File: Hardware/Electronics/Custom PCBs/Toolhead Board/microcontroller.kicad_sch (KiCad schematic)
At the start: 34 parts, among them J1 USB C Receptacle, J2 Conn_02x16_Odd_Even, J3 Conn_02x16_Odd_Even, J4 Conn_02x16_Odd_Even, J5 Conn_02x16_Odd_Even, SW1 BOOT, SW2 RESET, U3 RP2040, U4 W25Q128JVS, Y1 12MHz/12pF/50Ω/20ppm

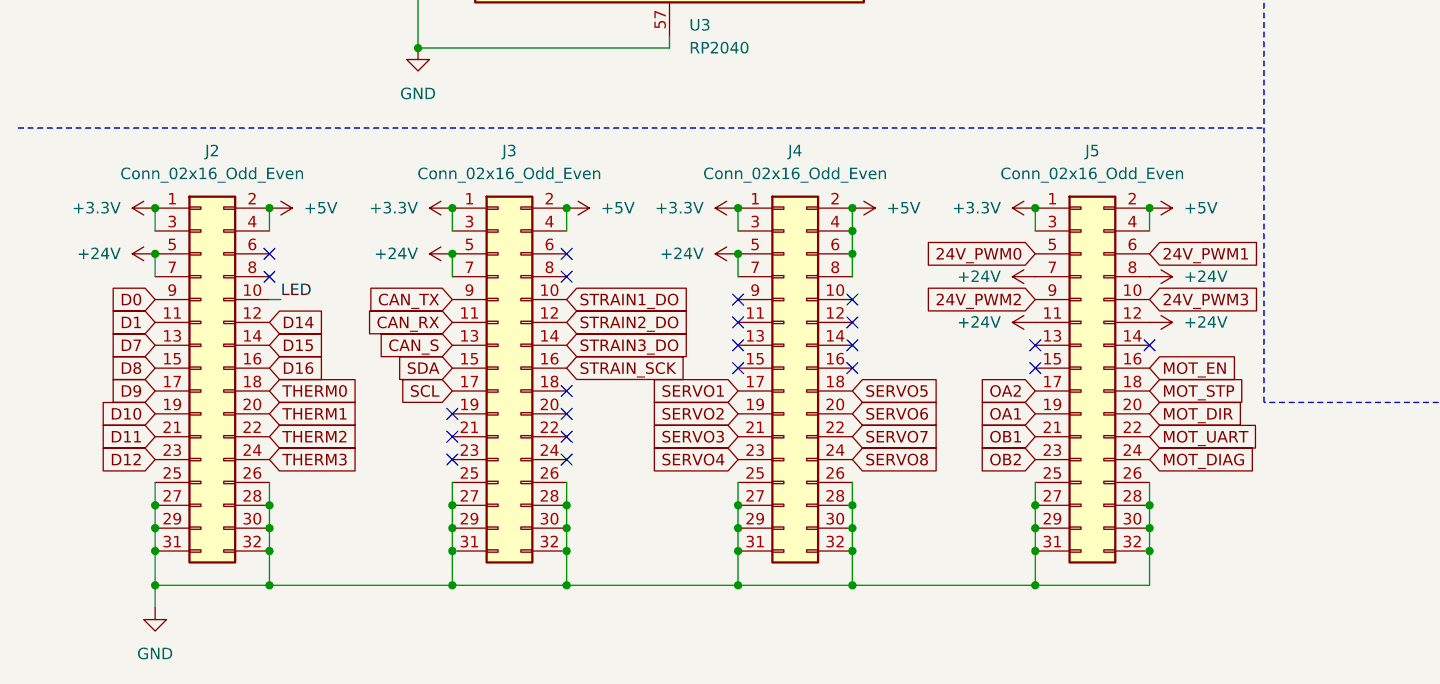
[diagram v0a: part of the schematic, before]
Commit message: Get basic Toolhead Board outline
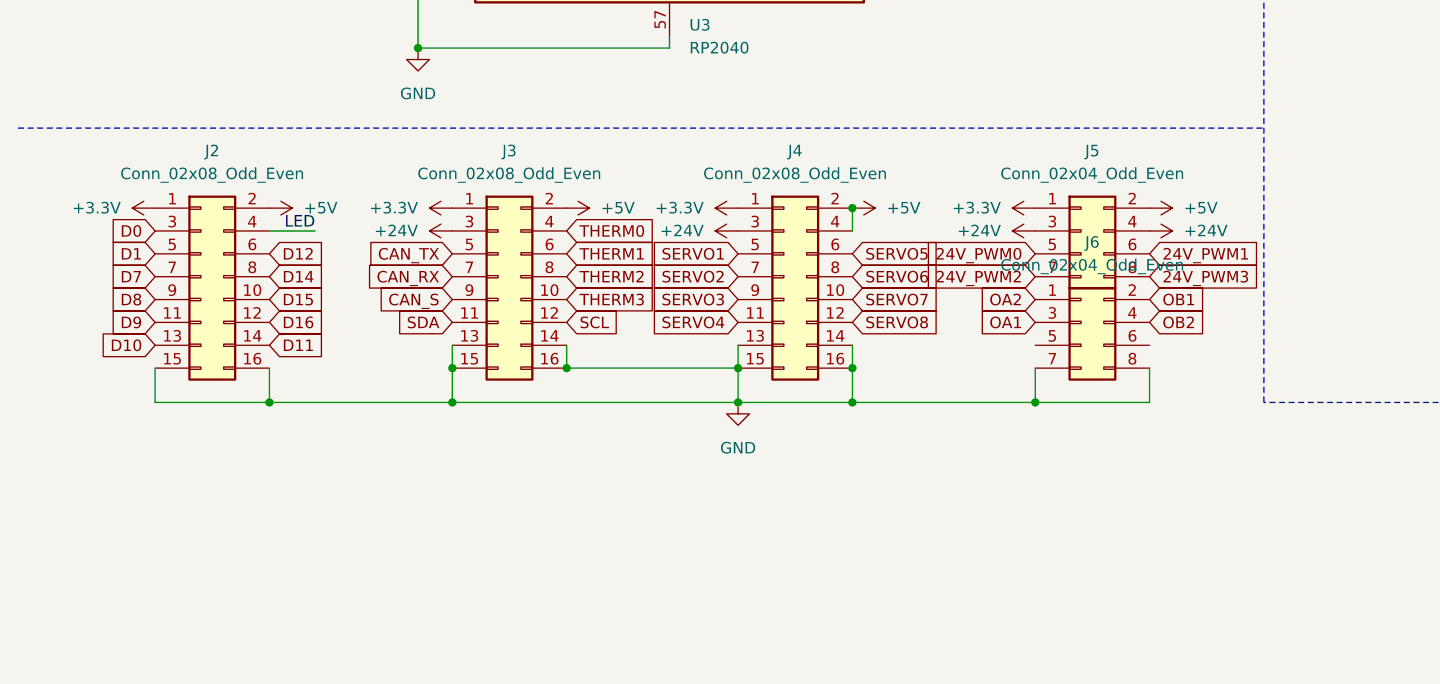
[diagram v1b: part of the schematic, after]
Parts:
- removed J2, J3, J4, J5: Conn_02x16_Odd_Even, Connector_PinHeader_2.54mm:PinHeader_2x16_P2.54mm_Vertical, symbol Connector_Generic:Conn_02x16_Odd_Even
- added J2, J3, J4: Conn_02x08_Odd_Even, Connector_PinSocket_2.54mm:PinSocket_2x08_P2.54mm_Vertical, symbol Connector_Generic:Conn_02x08_Odd_Even
- added J5, J6: Conn_02x04_Odd_Even, Connector_PinSocket_2.54mm:PinSocket_2x04_P2.54mm_Vertical, symbol Connector_Generic:Conn_02x04_Odd_Even
- J1: footprint usb_port:12402012E212A_AMP -> Connector_USB:USB_C_Receptacle_GCT_USB4105-xx-A_16P_TopMnt_Horizontal
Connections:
- net +24V: now also J3.3 (Pin_3), J4.3 (Pin_3), J5.3 (Pin_3), J5.4 (Pin_4)
- net +3.3V: now also J2.1 (Pin_1), J3.1 (Pin_1), J4.1 (Pin_1), J5.1 (Pin_1)
- net +5V: now also J2.2 (Pin_2), J3.2 (Pin_2), J4.2 (Pin_2), J4.4 (Pin_4), J5.2 (Pin_2)
- net 24V_PWM0: now also J5.5 (Pin_5)
- net 24V_PWM1: now also J5.6 (Pin_6)
- net 24V_PWM2: now also J5.7 (Pin_7)
- net 24V_PWM3: now also J5.8 (Pin_8)
- net CAN_RX: now also J3.7 (Pin_7)
- net CAN_S: now also J3.9 (Pin_9)
- net CAN_TX: now also J3.5 (Pin_5)
- net D0: now also J2.3 (Pin_3)
- net D1: now also J2.5 (Pin_5)
- net D10: now also J2.13 (Pin_13)
- net D11: now also J2.14 (Pin_14)
- net D12: now also J2.6 (Pin_6)
- net D14: now also J2.8 (Pin_8)
- net D15: now also J2.10 (Pin_10)
- net D16: now also J2.12 (Pin_12)
- net D7: now also J2.7 (Pin_7)
- net D8: now also J2.9 (Pin_9)
- net D9: now also J2.11 (Pin_11)
- net GND: now also J2.15 (Pin_15), J2.16 (Pin_16), J3.13 (Pin_13), J3.14 (Pin_14), J3.15 (Pin_15), J3.16 (Pin_16), J4.13 (Pin_13), J4.14 (Pin_14), J4.15 (Pin_15), J4.16 (Pin_16), J6.7 (Pin_7), J6.8 (Pin_8)
- net LED: now also J2.4 (Pin_4)
- net OA1: now also J6.3 (Pin_3)
- net OA2: now also J6.1 (Pin_1)
- net OB1: now also J6.2 (Pin_2)
- net OB2: now also J6.4 (Pin_4)
- net SCL: now also J3.12 (Pin_12)
- net SDA: now also J3.11 (Pin_11)
- net SERVO1: now also J4.5 (Pin_5)
- net SERVO2: now also J4.7 (Pin_7)
- net SERVO3: now also J4.9 (Pin_9)
- net SERVO4: now also J4.11 (Pin_11)
- net SERVO5: now also J4.6 (Pin_6)
- net SERVO6: now also J4.8 (Pin_8)
- net SERVO7: now also J4.10 (Pin_10)
- net SERVO8: now also J4.12 (Pin_12)
- net THERM0: now also J3.4 (Pin_4)
- net THERM1: now also J3.6 (Pin_6)
- net THERM2: now also J3.8 (Pin_8)
- net THERM3: now also J3.10 (Pin_10)
- no-connect marks 26 -> 4
